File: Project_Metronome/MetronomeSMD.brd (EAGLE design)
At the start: 62.4 x 31.5 mm, 45 parts

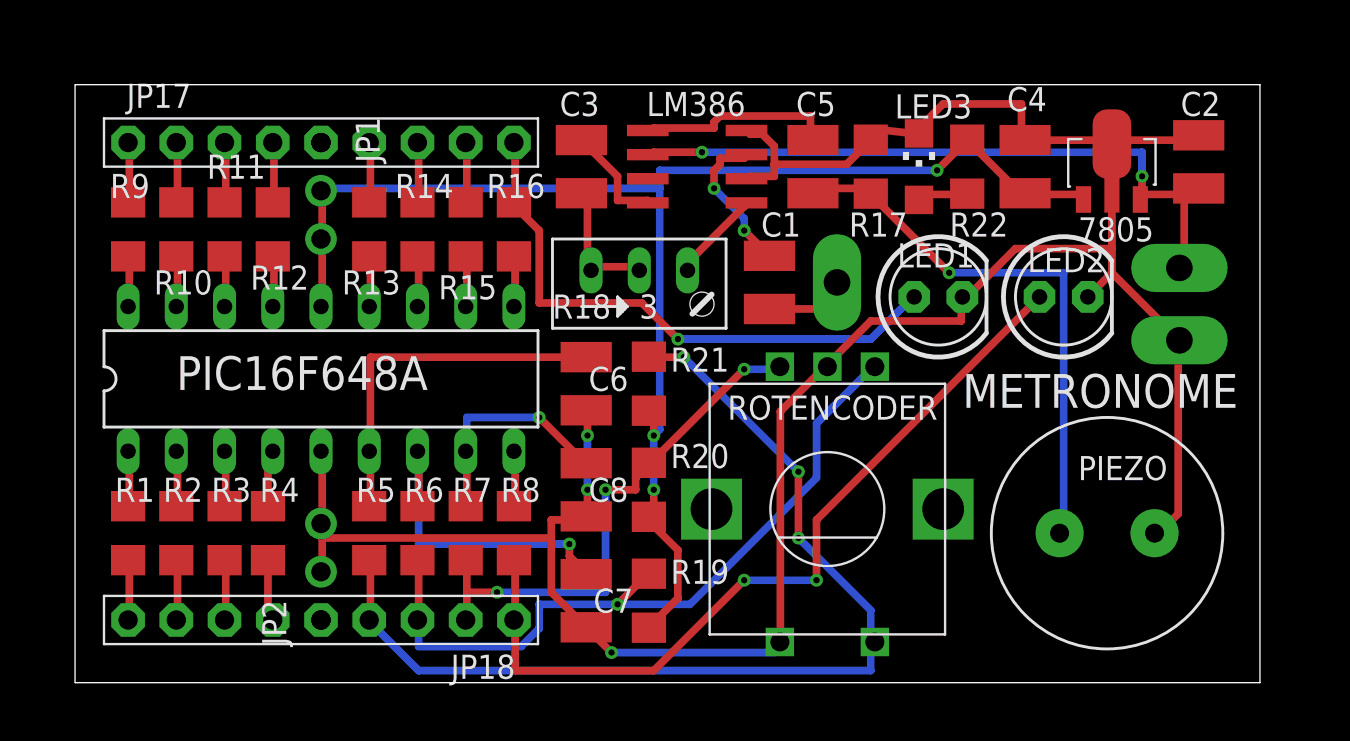
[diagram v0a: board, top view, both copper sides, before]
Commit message: better eagle files
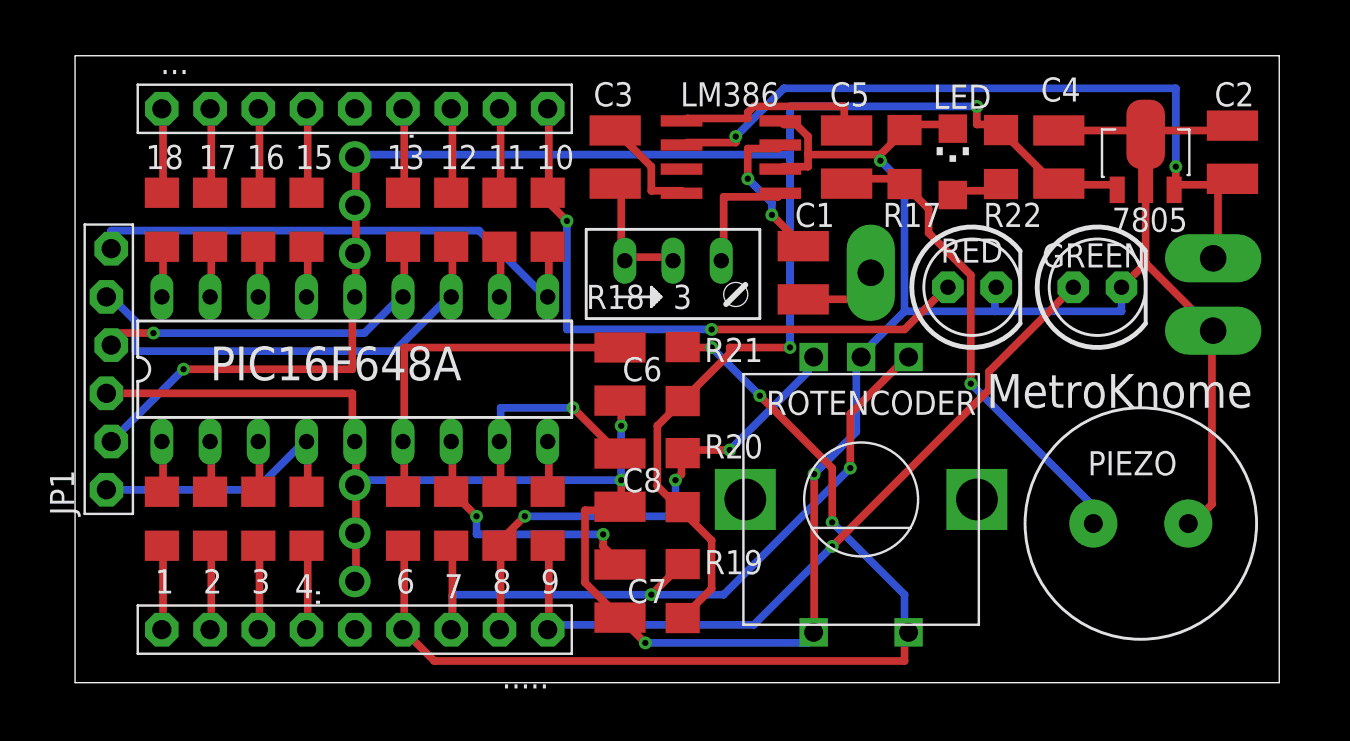
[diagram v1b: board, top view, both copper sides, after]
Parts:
- removed JP17, JP18: (no value), adafruit:1X09-BIG
- removed JP2: (no value), adafruit:1X03-CLEANBIG
- removed LED1: RED, adafruit:LED5MM
- removed LED2: GREEN, adafruit:LED5MM
- removed LED3: O, adafruit:CHIPLED_1206
- removed R1, R10, R11, R12, R13, R14, R15, R16, R2, R3, R4, R8, R9: 1k, resistor:R1206
- removed R5, R6, R7: 10k, resistor:R1206
- added ., ..: (no value), adafruit:1X03-CLEANBIG
- added ..., .....: (no value), adafruit:1X09-BIG
- added 1, 10, 11, 12, 13, 15, 16, 17, 18, 2, 3, 4, 9: 1k, resistor:R1206
- added 6, 7, 8: 10k, resistor:R1206
- added GREEN: GREEN, adafruit:LED5MM
- added LED: O, adafruit:CHIPLED_1206
- added RED: RED, adafruit:LED5MM
- JP1: device adafruit:1X03-CLEANBIG -> adafruit:1X06-BIGLOCK
- moved JP1 14.6 mm to (1.78, 16.5), turned to 90 degrees
- moved JP16 1.85 mm to (59.9, 18.5)
- moved C4 1.85 mm to (51.8, 27.7)
- moved JP9 1.85 mm to (59.9, 22.4)
- moved R17 1.85 mm to (43.7, 27.7)
- moved C6 1.85 mm to (28.7, 16.3)
- moved C7 1.85 mm to (28.7, 4.83)
- moved C8 1.85 mm to (28.7, 10.7)
- moved 7805 1.85 mm to (56.4, 27.9)
- moved C2 1.85 mm to (61.0, 27.9)
- moved PIC16F648A 1.85 mm to (14.7, 16.5)
- moved R21 1.85 mm to (32.0, 16.3)
- moved C1 1.85 mm to (38.4, 21.6)
- moved C3 1.85 mm to (28.4, 27.7)
- moved C5 1.85 mm to (40.6, 27.7)
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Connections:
- net GND: now also ...1, ...2, ...3, GREEN.K, JP1.3, LED.C, RED.K; no longer JP2.1, JP2.2, JP2.3, LED1.K, LED2.K, LED3.C
- net N$1: now also 9.2; no longer R8.2
- net N$10: now also ......9, 1.1; no longer JP18.9, R1.1
- net N$11: now also ......8, 2.1; no longer JP18.8, R2.1
- net N$12: now also ......7, 3.1; no longer JP18.7, R3.1
- net N$13: now also ......6, 4.1; no longer JP18.6, R4.1
- net N$14: now also ......4, 6.1; no longer JP18.4, R5.1
- net N$15: now also ......3, 7.1; no longer JP18.3, R6.1
- net N$16: now also ......2, 8.1; no longer JP18.2, R7.1
- net N$17: now also ......1, 9.1, GREEN.A; no longer JP18.1, LED2.A, R8.1
- net N$18: now also 18.1; no longer R9.1
- net N$19: now also 17.1; no longer R10.1
- net N$2: now also 1.2; no longer R1.2
- net N$20: now also 16.1; no longer R11.1
- net N$21: now also 15.1; no longer R12.1
- net N$22: now also 13.1, JP1.4; no longer R13.1
- net N$24: now also 12.1, JP1.5; no longer R14.1
- net N$26: now also 11.1; no longer R15.1
- net N$27: now also 10.1, JP1.6; no longer R16.1
- net N$28: now also ....1, 18.2; no longer JP17.1, R9.2
- net N$29: now also ....2, 17.2; no longer JP17.2, R10.2
- net N$3: now also 2.2; no longer R2.2
- net N$30: now also ....3, 16.2; no longer JP17.3, R11.2
- net N$31: now also ....4, 15.2; no longer JP17.4, R12.2
- net N$32: now also ....6, 13.2; no longer JP17.6, R13.2
- net N$34: now also ....7, 12.2; no longer JP17.7, R14.2
- net N$37: now also ....8, 11.2; no longer JP17.8, R15.2
- net N$38: now also ....9, 10.2, RED.A; no longer JP17.9, LED1.A, R16.2
- net N$4: now also 3.2; no longer R3.2
- net N$40: now also LED.A; no longer LED3.A
- net N$5: now also 4.2, JP1.1; no longer R4.2
- net N$6: now also 6.2; no longer R5.2
- net N$7: now also 7.2; no longer R6.2
- net N$8: now also 8.2; no longer R7.2
- net VDD: now also ..1, ..2, ..3; no longer JP1.1, JP1.3
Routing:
- net VDD: track 76.1 -> 102.9 mm
- net N$27: track 2.66 -> 28.0 mm
- net N$24: track 2.66 -> 24.1 mm
- net GND: track 134.6 -> 152.4 mm, vias 3 -> 5
- net N$22: track 2.66 -> 19.5 mm, vias 0 -> 1
- net N$5: track 3.05 -> 14.3 mm
- net VCC: track 36.9 -> 41.2 mm
- net N$39: track 29.8 -> 26.0 mm
- net N$7: track 17.7 -> 14.1 mm, vias 1 -> 2
- net N$17: track 43.5 -> 40.3 mm, vias 2 -> 1
- net N$38: track 30.5 -> 33.0 mm, vias 1 -> 2
- net N$25: track 4.81 -> 6.49 mm
- net N$12: track 3.18 -> 4.46 mm
- net N$10: track 3.18 -> 4.46 mm
- net N$11: track 3.18 -> 4.46 mm
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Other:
- board size 62.4 x 31.5 mm -> 63.4 x 33 mm
- board text added: "METROKNOME_2016"
- board text added: "MetroKnome"
- board text removed: "METRONOME"
- board text removed: "METRONOME_2016"
